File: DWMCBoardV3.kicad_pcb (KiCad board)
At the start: 2 copper layers, 32.5 x 19.5 mm, 7 parts, among them J1 Battery, J2 TPL5110, J3 MCU, Q1 S8050

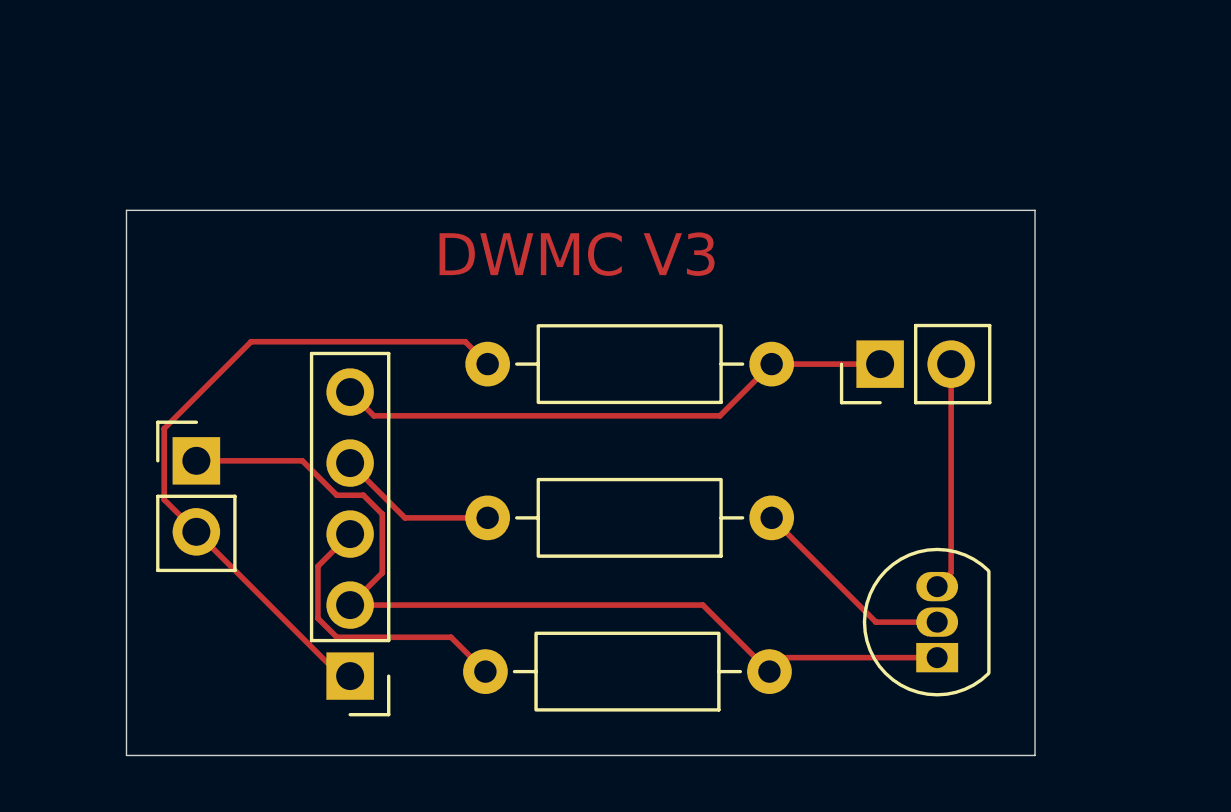
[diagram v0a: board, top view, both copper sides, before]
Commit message: Add files via upload
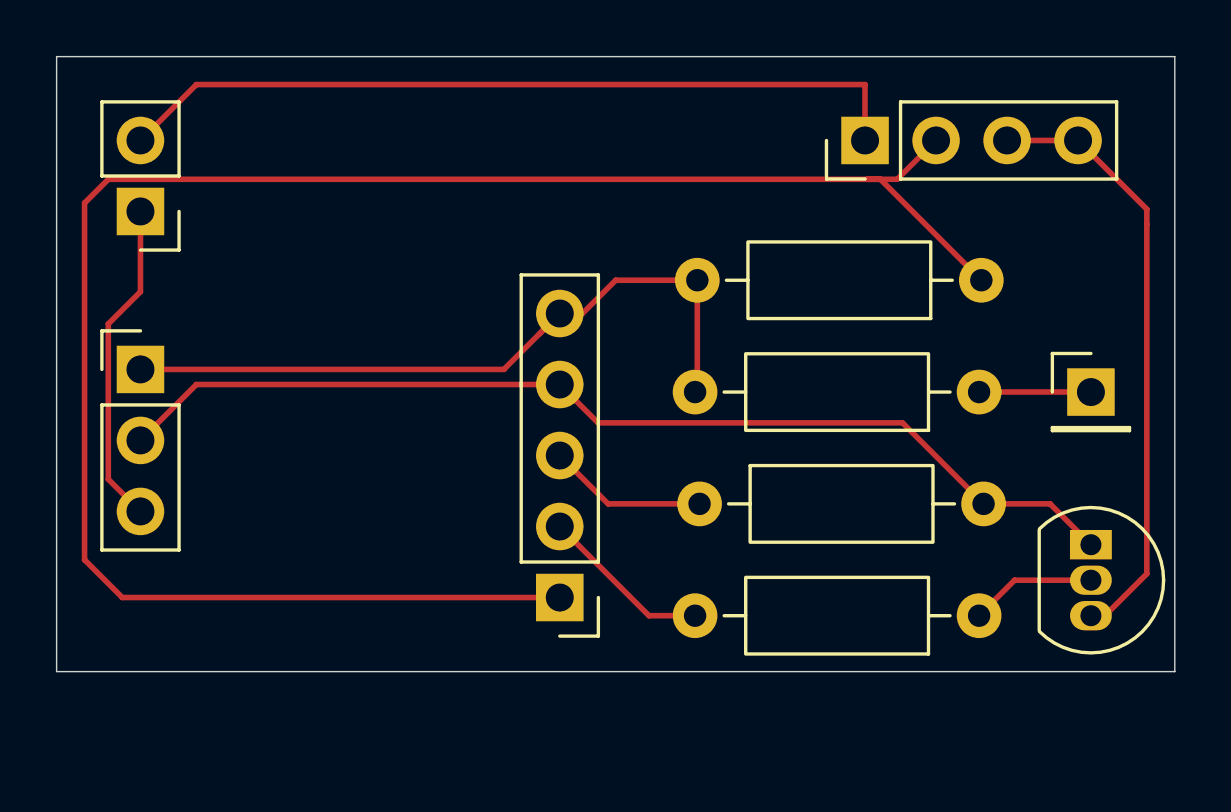
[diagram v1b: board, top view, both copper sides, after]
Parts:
- added J4: Conn_01x02, Connector_PinHeader_2.54mm:PinHeader_1x02_P2.54mm_Vertical, F.Cu at (43.0, 83.5)
- added J5: Therm, Connector_PinHeader_2.54mm:PinHeader_1x01_P2.54mm_Vertical, F.Cu at (77.0, 90.0)
- added R4: 10K, Resistor_THT:R_Axial_DIN0207_L6.3mm_D2.5mm_P10.16mm_Horizontal, F.Cu at (73.0, 90.0)
- J1: footprint Connector_PinHeader_2.54mm:PinHeader_1x02_P2.54mm_Vertical -> Connector_PinHeader_2.54mm:PinHeader_1x03_P2.54mm_Vertical
- J3: value MCU -> Conn_01x04; footprint Connector_PinHeader_2.54mm:PinHeader_1x02_P2.54mm_Vertical -> Connector_PinHeader_2.54mm:PinHeader_1x04_P2.54mm_Vertical
- moved R2 8.20 mm to (73.0, 98.0)
- moved R1 8.08 mm to (73.1, 86.0)
- moved J3 8.02 mm to (68.9, 81.0)
- moved J2 8.01 mm to (58.0, 97.3)
- moved Q1 6.82 mm to (77.0, 95.5), turned to -90 degrees
- moved R3 6.50 mm to (63.0, 94.0), turned to 0 degrees
- moved J1 3.83 mm to (43.0, 89.2)
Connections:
- J1 pad 1: GND1 -> Net-(J1-Pin_1)
- J1 pad 2: Net-(J1-Pin_2) -> GND
- J2 pad 1: Net-(J1-Pin_2) -> Net-(J2-Pin_1)
- J2 pad 2: GND1 -> Net-(J2-Pin_2)
- J2 pad 4: Net-(J2-Pin_4) -> GND
- J2 pad 5: Net-(J2-Pin_5) -> Net-(J1-Pin_1)
- J3 pad 1: Net-(J2-Pin_5) -> Net-(J3-Pin_1)
- J3 pad 2: Net-(J3-Pin_2) -> Net-(J2-Pin_1)
- Q1 pad 1: GND1 -> GND
- Q1 pad 3: Net-(J3-Pin_2) -> Net-(J3-Pin_3)
- R1 pad 1: Net-(J2-Pin_5) -> Net-(J2-Pin_1)
- R1 pad 2: Net-(J1-Pin_2) -> Net-(J1-Pin_1)
- R2 pad 2: Net-(J2-Pin_4) -> Net-(J2-Pin_2)
- R3 pad 1: GND1 -> Net-(J2-Pin_3)
- R3 pad 2: Net-(J2-Pin_3) -> GND
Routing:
- net Net-(J2-Pin_1): track 0.00 -> 67.9 mm
- net GND: track 0.00 -> 37.2 mm
- net GND1: track 33.9 -> 0.00 mm
- net Net-(J3-Pin_1): track 0.00 -> 28.7 mm
- net Net-(J1-Pin_1): track 0.00 -> 26.3 mm
- net Net-(J1-Pin_2): track 25.0 -> 0.00 mm
- net Net-(J3-Pin_3): track 0.00 -> 21.7 mm
- net Net-(J2-Pin_5): track 20.2 -> 0.00 mm
- net Net-(J1-Pin_3): track 0.00 -> 11.7 mm
- net Net-(J3-Pin_2): track 8.54 -> 0.00 mm
- net Net-(J2-Pin_2): track 0.00 -> 6.16 mm
- net Net-(J2-Pin_4): track 5.84 -> 0.00 mm
- net Net-(J2-Pin_3): track 10.3 -> 5.72 mm
- net Net-(J5-Pin_1): track 0.00 -> 4.00 mm
- net Net-(Q1-B): track 7.47 -> 4.53 mm
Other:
- board size 32.5 x 19.5 mm -> 40 x 22 mm
- board text removed: "DWMC V3"
